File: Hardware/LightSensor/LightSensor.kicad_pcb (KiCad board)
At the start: 2 copper layers, 18 x 13 mm, 7 parts, among them J1 Conn_01x04_Pin, U1 VEML6040

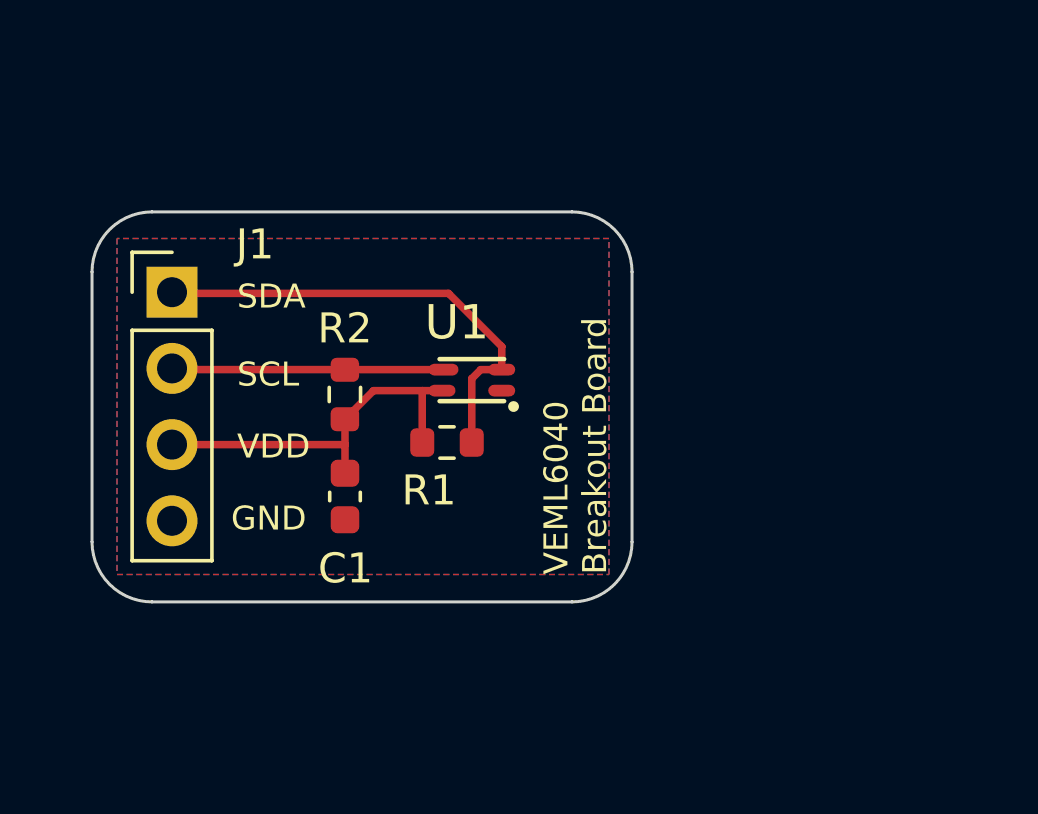
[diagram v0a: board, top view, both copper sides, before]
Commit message: $1
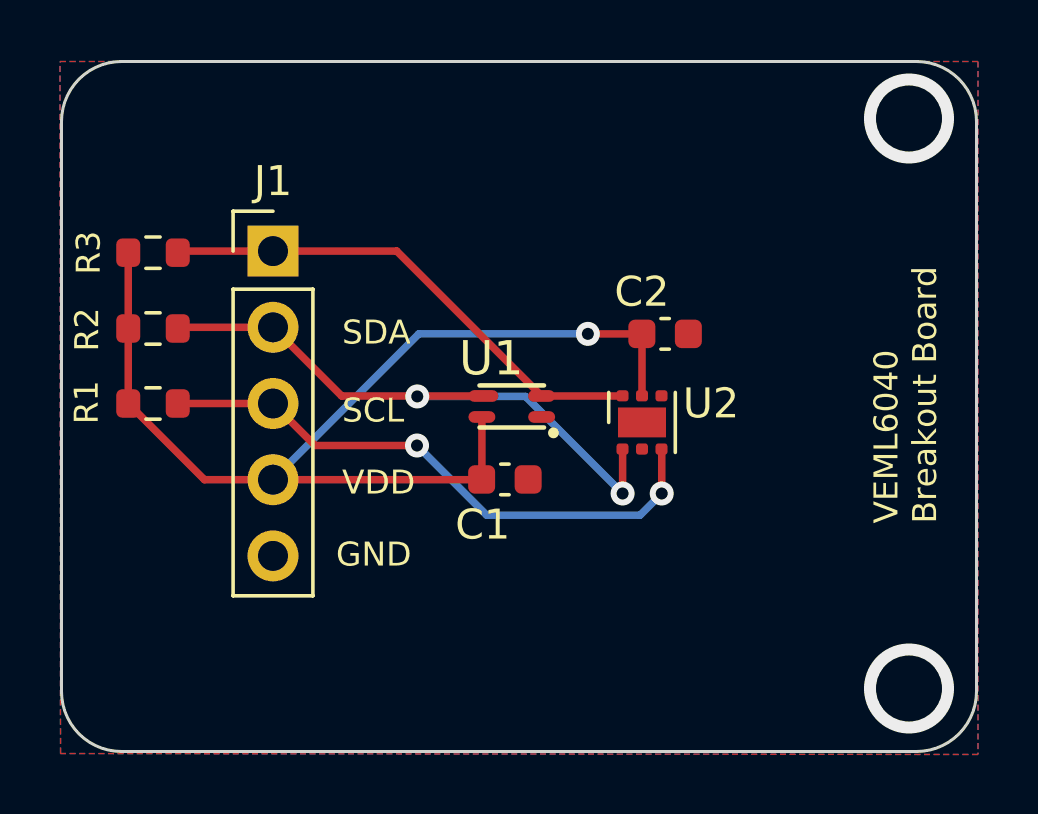
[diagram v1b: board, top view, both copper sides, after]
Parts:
- added C2: 100n, Capacitor_SMD:C_0603_1608Metric, F.Cu at (226.9, 110.8)
- added R3: 4.7k, Resistor_SMD:R_0603_1608Metric, F.Cu at (209.8, 108.1)
- added U2: TMP116xxDRV, Package_SON:WSON-6-1EP_2x2mm_P0.65mm_EP1x1.6mm, F.Cu at (226.1, 113.7)
- J1: footprint Connector_PinHeader_2.54mm:PinHeader_1x04_P2.54mm_Vertical -> Connector_PinHeader_2.54mm:PinHeader_1x05_P2.54mm_Vertical
- moved G*** 13.7 mm to (224.6, 104.5)
- moved R1 9.89 mm to (209.8, 113.1)
- moved G*** 6.83 mm to (213.5, 104.0)
- moved R2 6.76 mm to (209.8, 110.6), turned to 0 degrees
- moved C1 5.36 mm to (221.5, 115.6), turned to 180 degrees
- moved J1 3.63 mm to (213.8, 108.0)
- moved U1 1.59 mm to (221.8, 113.2)
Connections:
- J1 pad 3: /+3.3V -> /ALERT
- J1 pad 4: GND -> /+3.3V
- R1 pad 2: /SDA -> /ALERT
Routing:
- net /+3.3V: track 12.9 -> 36.3 mm, vias 0 -> 1
- net /ALERT: track 0.00 -> 19.5 mm, vias 0 -> 2
- net /SCL: track 9.08 -> 20.8 mm, vias 0 -> 2
- net /SDA: track 15.8 -> 16.9 mm
- net (no net): vias 0 -> 2
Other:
- board size 18 x 13 mm -> 30.5 x 23 mm
